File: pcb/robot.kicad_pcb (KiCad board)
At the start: 2 copper layers, 50.2 x 48.3 mm, 20 parts, among them J1 MA, J2 MB, J3 Conn_01x03, J4 Conn_01x03, J5 BATT, J6 BATT, J7 STBY, J8 PWR 5V, J9 PWR 3V3, U1 TB6612FNG, U2 L7805, U3 L78L33_TO92

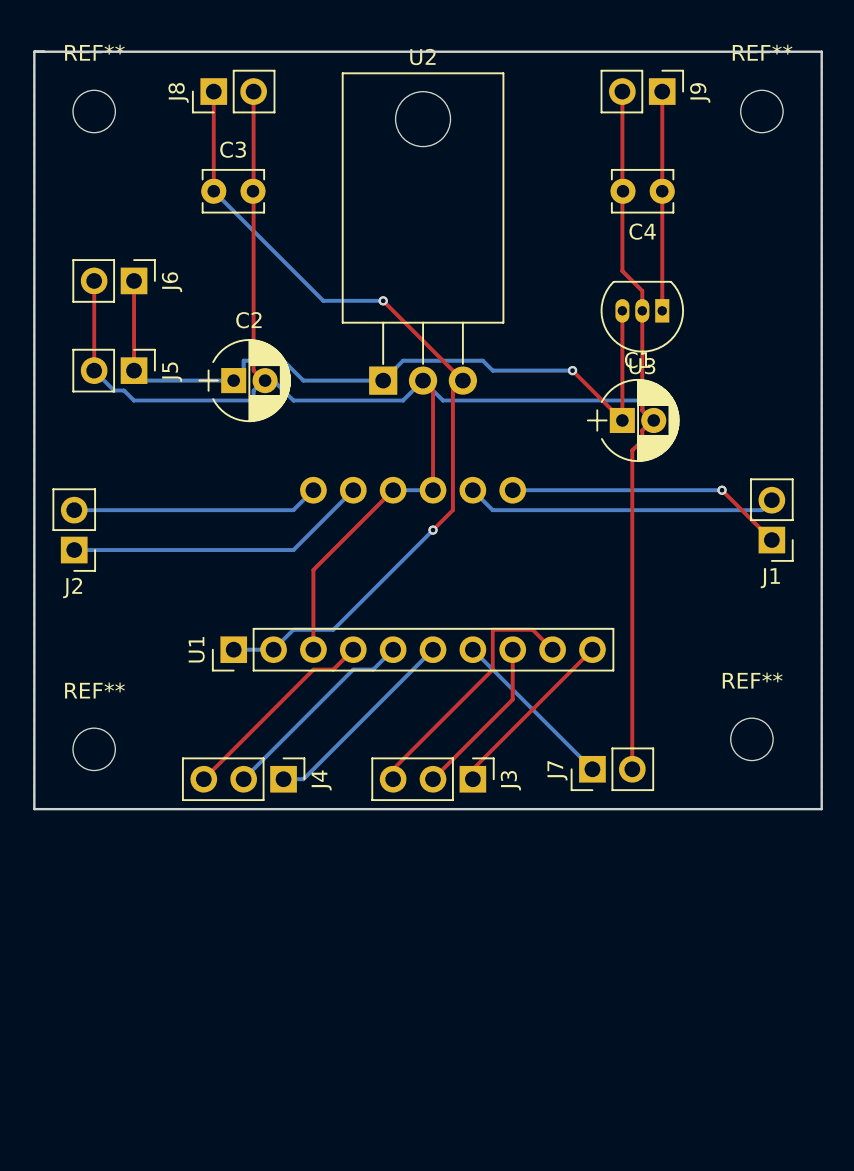
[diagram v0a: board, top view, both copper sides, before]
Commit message: updates
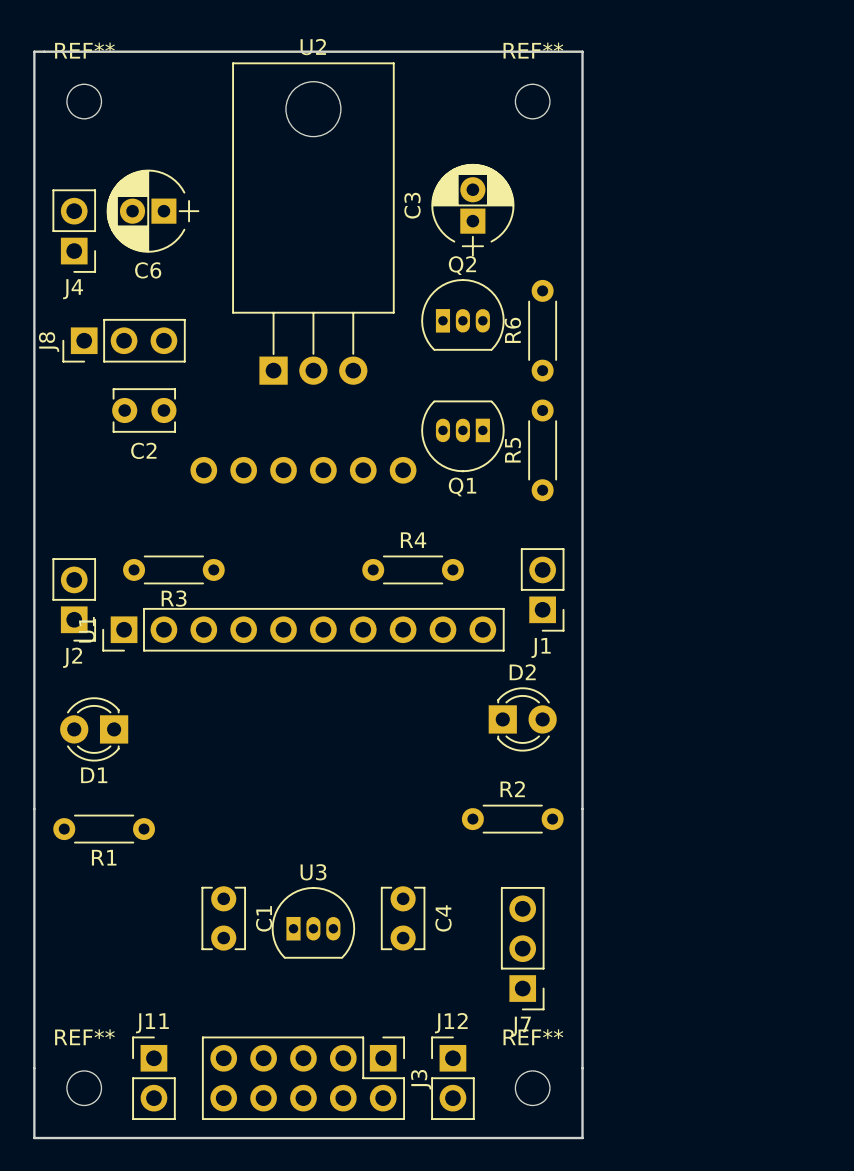
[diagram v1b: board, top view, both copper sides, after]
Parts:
- removed J5, J6: BATT, Pin_Headers:Pin_Header_Straight_1x02_Pitch2.54mm
- removed J9: PWR 3V3, Pin_Headers:Pin_Header_Straight_1x02_Pitch2.54mm
- removed the REF** at (142.2, 33.0)
- removed the REF** at (99.7, 33.0)
- removed the REF** at (99.7, 73.7)
- removed the REF** at (141.6, 73.0)
- added C6: 33uF, Capacitors_THT:CP_Radial_D5.0mm_P2.00mm, F.Cu at (104.1, 39.4)
- added D1: PWR, LEDs:LED_D3.0mm, F.Cu at (101.0, 72.4)
- added D2: STBY, LEDs:LED_D3.0mm, F.Cu at (125.7, 71.8)
- added J11: MB CTRL, Pin_Headers:Pin_Header_Straight_1x02_Pitch2.54mm, F.Cu at (103.5, 93.3)
- added J12: MA CTRL, Pin_Headers:Pin_Header_Straight_1x02_Pitch2.54mm, F.Cu at (122.6, 93.3)
- added Q1: PN2222A, TO_SOT_Packages_THT:TO-92_Inline_Narrow_Oval, F.Cu at (124.5, 53.3)
- added Q2: PN2222A, TO_SOT_Packages_THT:TO-92_Inline_Narrow_Oval, F.Cu at (121.9, 46.4)
- added R1: 330, Resistors_THT:R_Axial_DIN0204_L3.6mm_D1.6mm_P5.08mm_Horizontal, F.Cu at (102.9, 78.7)
- added R2: 330, Resistors_THT:R_Axial_DIN0204_L3.6mm_D1.6mm_P5.08mm_Horizontal, F.Cu at (123.8, 78.1)
- added R3: 10k, Resistors_THT:R_Axial_DIN0204_L3.6mm_D1.6mm_P5.08mm_Horizontal, F.Cu at (107.3, 62.2)
- added R4: 10k, Resistors_THT:R_Axial_DIN0204_L3.6mm_D1.6mm_P5.08mm_Horizontal, F.Cu at (117.5, 62.2)
- added R5: 10k, Resistors_THT:R_Axial_DIN0204_L3.6mm_D1.6mm_P5.08mm_Horizontal, F.Cu at (128.3, 57.1)
- added R6: 10k, Resistors_THT:R_Axial_DIN0204_L3.6mm_D1.6mm_P5.08mm_Horizontal, F.Cu at (128.3, 49.5)
- added REF**: MountingHole_2.2mm_M2, Mounting_Holes:MountingHole_2.2mm_M2, F.Cu at (127.6, 32.4)
- added REF**: MountingHole_2.2mm_M2, Mounting_Holes:MountingHole_2.2mm_M2, F.Cu at (99.1, 32.4)
- added REF**: MountingHole_2.2mm_M2, Mounting_Holes:MountingHole_2.2mm_M2, F.Cu at (127.6, 95.2)
- added REF**: MountingHole_2.2mm_M2, Mounting_Holes:MountingHole_2.2mm_M2, F.Cu at (99.1, 95.2)
- C1, C2: value CP -> 0.1uF; footprint Capacitors_THT:CP_Radial_D5.0mm_P2.00mm -> Capacitors_THT:C_Disc_D3.8mm_W2.6mm_P2.50mm
- C3: value C_Small -> 10uF; footprint Capacitors_THT:C_Disc_D3.8mm_W2.6mm_P2.50mm -> Capacitors_THT:CP_Radial_D5.0mm_P2.00mm
- C4: value C_Small -> 0.1uF
- J1: value MA -> MA PWR
- J2: value MB -> MB PWR
- J3: value Conn_01x03 -> Power Connector; footprint Pin_Headers:Pin_Header_Straight_1x03_Pitch2.54mm -> Pin_Headers:Pin_Header_Straight_2x05_Pitch2.54mm
- J4: value Conn_01x03 -> BATT; footprint Pin_Headers:Pin_Header_Straight_1x03_Pitch2.54mm -> Pin_Headers:Pin_Header_Straight_1x02_Pitch2.54mm
- J7: footprint Pin_Headers:Pin_Header_Straight_1x02_Pitch2.54mm -> Pin_Headers:Pin_Header_Straight_1x03_Pitch2.54mm
- J8: value PWR 5V -> PWR; footprint Pin_Headers:Pin_Header_Straight_1x02_Pitch2.54mm -> Pin_Headers:Pin_Header_Straight_1x03_Pitch2.54mm
- moved C4 48.0 mm to (119.4, 83.2), turned to 270 degrees
- moved U3 45.8 mm to (112.4, 85.1), turned to 0 degrees
- moved C1 39.7 mm to (108.0, 83.2), turned to 270 degrees
- moved J4 36.2 mm to (98.4, 41.9), turned to 180 degrees
- moved J3 18.7 mm to (118.1, 93.3)
- moved J8 17.9 mm to (99.1, 47.6)
- moved C3 16.6 mm to (123.8, 40.0), turned to 90 degrees
- moved J1 15.3 mm to (128.3, 64.8)
- moved J7 14.7 mm to (127.0, 88.9), turned to 180 degrees
- moved U1 7.10 mm to (101.6, 66.0)
- moved U2 7.01 mm to (111.1, 49.5)
- moved C2 4.84 mm to (104.1, 52.1), turned to 180 degrees
- moved J2 4.45 mm to (98.4, 65.4)
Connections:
- C1 pad 1: +BATT -> +5V
- C2 pad 1: +BATT -> VCC
- J3 pad 1: Net-(J3-Pad1) -> VCC
- J3 pad 2: Net-(J3-Pad2) -> VCC
- J3 pad 3: Net-(J3-Pad3) -> +5V
- J4 pad 1: Net-(J4-Pad1) -> +BATT
- J4 pad 2: Net-(J4-Pad2) -> GND
- J7 pad 2: GND -> +3V3
- J8 pad 1: +5V -> (no net)
- J8 pad 2: GND -> +BATT
- U1 pad 10: Net-(J3-Pad1) -> APWM
- U1 pad 15: Net-(J1-Pad2) -> Net-(J1-Pad1)
- U1 pad 16: Net-(J1-Pad1) -> Net-(J1-Pad2)
- U1 pad 4: Net-(J4-Pad3) -> BPWM
- U1 pad 5: Net-(J4-Pad2) -> B2
- U1 pad 6: Net-(J4-Pad1) -> B1
- U1 pad 8: Net-(J3-Pad2) -> A2
- U1 pad 9: Net-(J3-Pad3) -> A1
- U2 pad 1: +BATT -> VCC
- U3 pad 3: +BATT -> +5V
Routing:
- net GND: track 131.2 -> 0.00 mm
- net +5V: track 53.4 -> 0.00 mm, vias 2 -> 0
- net +BATT: track 47.6 -> 0.00 mm, vias 1 -> 0
- net Net-(J1-Pad2): track 19.8 -> 0.00 mm
- net Net-(J2-Pad1): track 19.4 -> 0.00 mm
- net Net-(J1-Pad1): track 17.8 -> 0.00 mm, vias 1 -> 0
- net Net-(J3-Pad3): track 16.5 -> 0.00 mm
- net Net-(J2-Pad2): track 15.8 -> 0.00 mm
- net +3V3: track 14.0 -> 0.00 mm
- net Net-(J4-Pad2): track 12.9 -> 0.00 mm
- net Net-(J4-Pad3): track 12.9 -> 0.00 mm
- net Net-(J4-Pad1): track 12.9 -> 0.00 mm
- net Net-(J3-Pad1): track 11.4 -> 0.00 mm
- net STBY: track 10.8 -> 0.00 mm
- net Net-(J3-Pad2): track 10.4 -> 0.00 mm
- removed copper zone on B.Cu, net GND
- removed copper zone on F.Cu, net GND
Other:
- board size 50.2 x 48.3 mm -> 34.9 x 69.2 mm
- net class power added: clearance 0.2, trace_width 0.25, via_dia 0.6, via_drill 0.4
